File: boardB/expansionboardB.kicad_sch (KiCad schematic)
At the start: 38 parts, among them J1 USB_C_Receptacle, J3 HDMI_A, SW3 ESPRESET, SW4 ESPPROG, U1 ESP32-S3-WROOM-1, U2 GPIO_U2, U4 GPIO_U4, U5 SII1136CTU, U7 MAX20022ATIA+T

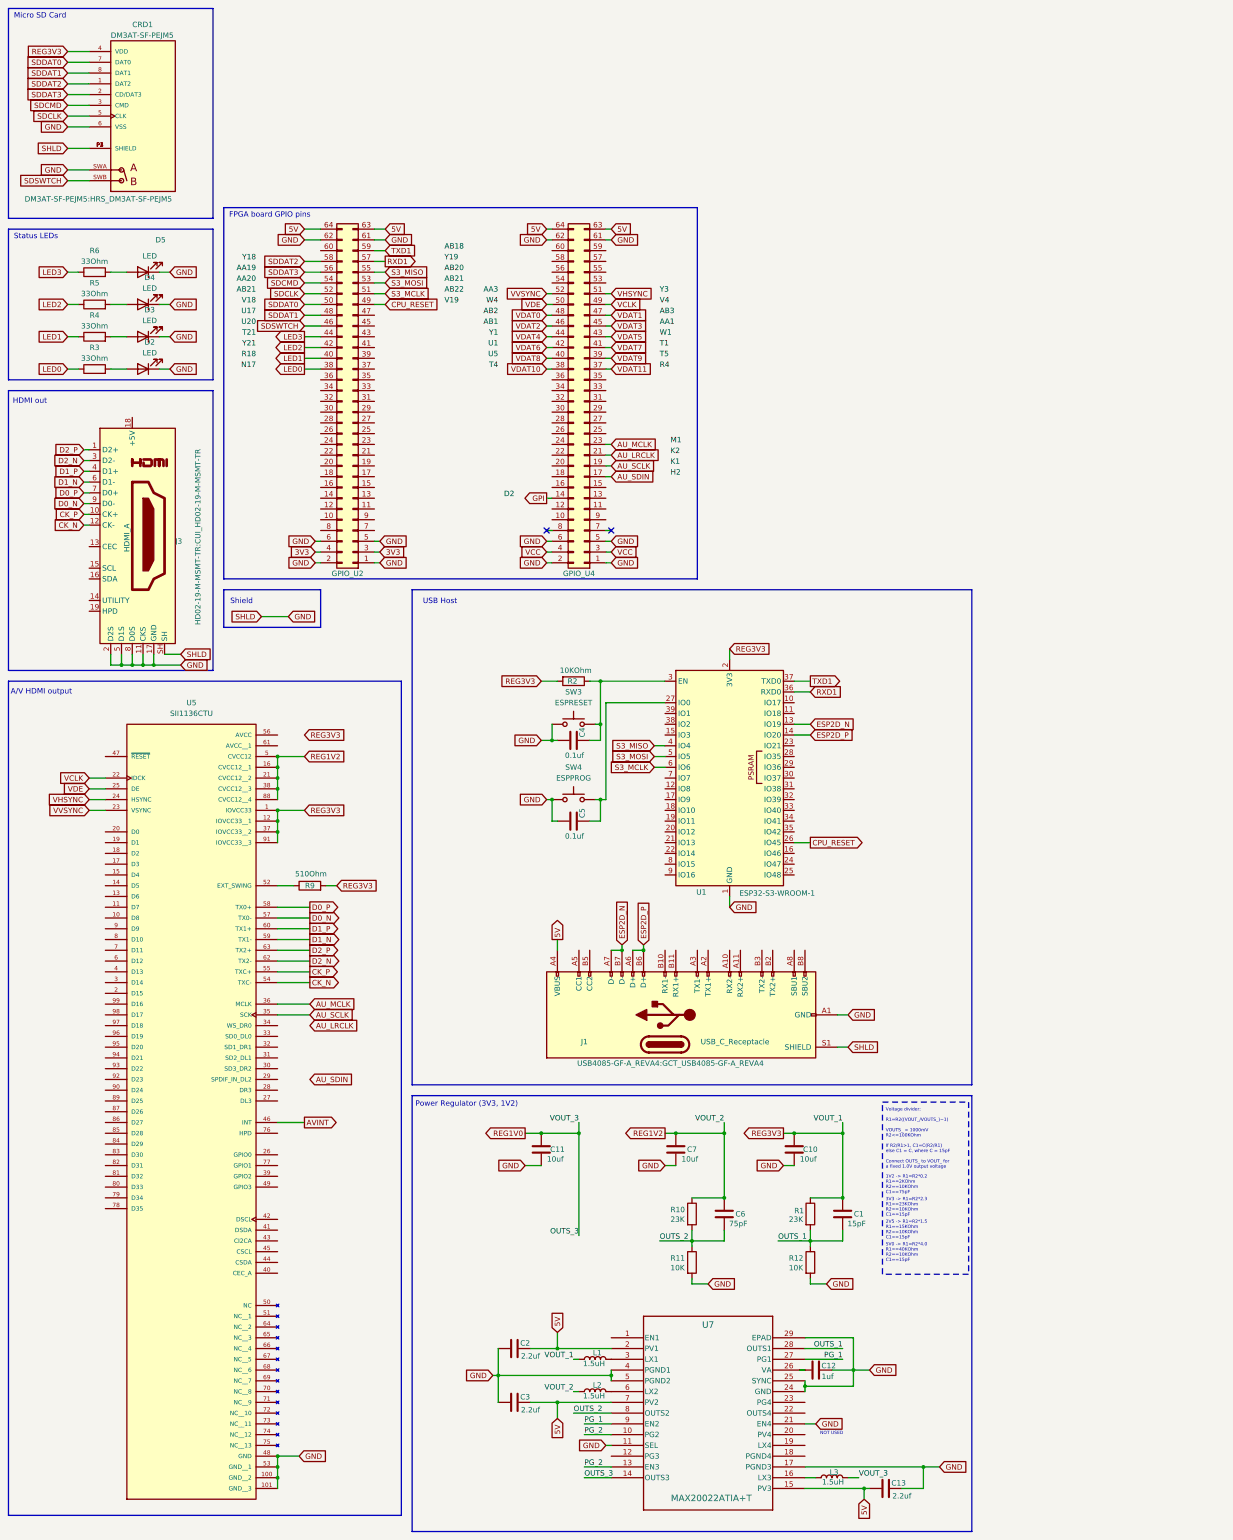
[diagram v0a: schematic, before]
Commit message: Updated new board
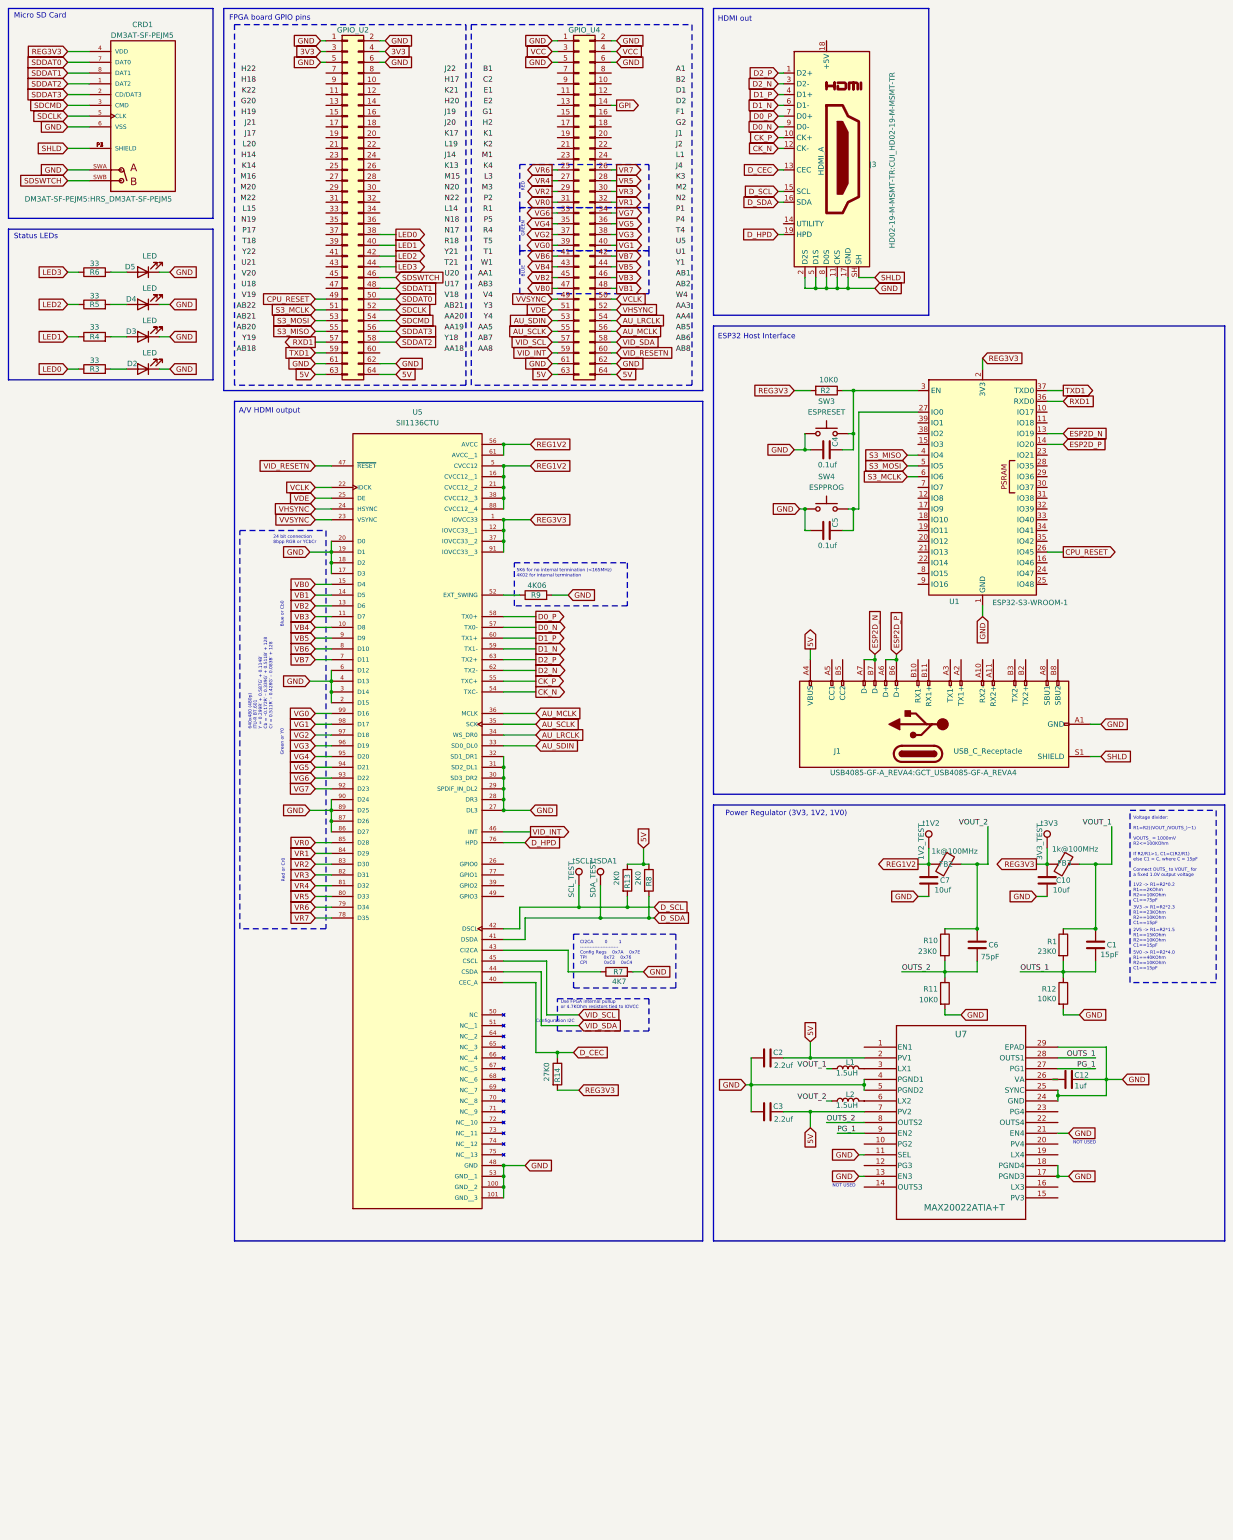
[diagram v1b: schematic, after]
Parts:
- removed C11: 10uf, Capacitor_SMD:C_0603_1608Metric_Pad1.08x0.95mm_HandSolder, symbol Device:C
- removed C13: 2.2uf, Capacitor_SMD:C_0603_1608Metric_Pad1.08x0.95mm_HandSolder, symbol Device:C
- removed L3: 1.5uH, Inductor_SMD:L_0805_2012Metric, symbol Device:L
- added FB2, FB3: 1k@100MHz, Resistor_SMD:R_0805_2012Metric_Pad1.20x1.40mm_HandSolder, symbol graphics-card-rev-2-rescue:Ferrite_Bead-Device
- added R13, R8: 2K0, Resistor_SMD:R_0603_1608Metric_Pad0.98x0.95mm_HandSolder, symbol Device:R
- added R14: 27K0, Resistor_SMD:R_0603_1608Metric_Pad0.98x0.95mm_HandSolder, symbol Device:R
- added R7: 4K7, Resistor_SMD:R_0603_1608Metric_Pad0.98x0.95mm_HandSolder, symbol Device:R
- added t1V2: 1V2_TEST, TestPoint:TestPoint_Pad_D1.5mm, symbol Connector:TestPoint
- added t3V3: 3V3_TEST, TestPoint:TestPoint_Pad_D1.5mm, symbol Connector:TestPoint
- added tSCL1: SCL_TEST, TestPoint:TestPoint_Pad_D1.5mm, symbol Connector:TestPoint
- added tSDA1: SDA_TEST, TestPoint:TestPoint_Pad_D1.5mm, symbol Connector:TestPoint
- R1, R10: value 23K -> 23K0
- R11, R12: value 10K -> 10K0
- R2: value 10KOhm -> 10K0
- R3, R4, R5, R6: value 33Ohm -> 33
- R9: value 510Ohm -> 4K06
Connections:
- net AVINT is gone; now on net VID_INT: U5.46 (INT)
- net VDAT0 is gone; now on net VB1: U4.48 (Pin_48)
- net VDAT1 is gone; now on net VB0: U4.47 (Pin_47)
- net VDAT10 is gone; now on net VG3: U4.38 (Pin_38)
- net VDAT11 is gone; now on net VG2: U4.37 (Pin_37)
- net VDAT2 is gone; now on net VB3: U4.46 (Pin_46)
- net VDAT3 is gone; now on net VB2: U4.45 (Pin_45)
- net VDAT4 is gone; now on net VB5: U4.44 (Pin_44)
- net VDAT5 is gone; now on net VB4: U4.43 (Pin_43)
- net VDAT6 is gone; now on net VB7: U4.42 (Pin_42)
- net VDAT7 is gone; now on net VB6: U4.41 (Pin_41)
- net VDAT8 is gone; now on net VG1: U4.40 (Pin_40)
- net VDAT9 is gone; now on net VG0: U4.39 (Pin_39)
- net 5V: now also R13.1, R8.1; no longer U7.15 (PV3)
- net AU_LRCLK: now also U4.54 (Pin_54), U5.34 (WS_DR0); no longer U4.21 (Pin_21)
- net AU_MCLK: now also U4.56 (Pin_56); no longer U4.23 (Pin_23)
- net AU_SCLK: now also U4.55 (Pin_55); no longer U4.19 (Pin_19)
- net AU_SDIN: now also U4.53 (Pin_53), U5.33 (SD0_DL0); no longer U4.17 (Pin_17)
- net GND: now also R9.2, U5.17 (D3), U5.18 (D2), U5.19 (D1), U5.2 (D15), U5.20 (D0), U5.27 (DL3), U5.28 (DR3), U5.29 (SPDIF_IN_DL2), U5.3 (D14), U5.30 (SD3_DR2), U5.31 (SD2_DL1), U5.32 (SD1_DR1), U5.4 (D13), U5.6 (D12), U5.86 (D27), U5.87 (D26), U5.89 (D25), U5.90 (D24), U7.13 (EN3), U7.18 (PGND4), R7.2; no longer CRD1.P1 (SHIELD), CRD1.P2 (SHIELD), CRD1.P3 (SHIELD), CRD1.P4 (SHIELD), J1.S1 (SHIELD), J3.SH
- net REG1V2: now also U5.56 (AVCC), U5.61 (AVCC__1), FB2.2, t1V2.1; no longer C6.1, L2.1, R10.1
- net REG3V3: now also FB3.2, R14.2, t3V3.1; no longer C1.1, L1.1, R1.1, R9.2
- net VCLK: now also U4.50 (Pin_50); no longer U4.49 (Pin_49)
- net VDE: now also U4.51 (Pin_51); no longer U4.50 (Pin_50)
- net VHSYNC: now also U4.52 (Pin_52); no longer U4.51 (Pin_51)
- net VVSYNC: now also U4.49 (Pin_49); no longer U4.52 (Pin_52)
- net VR6: now reaches U4.25 (Pin_25)
- net VR6: now also U5.79 (D34)
- net VR7: now reaches U4.26 (Pin_26)
- net VR7: now also U5.78 (D35)
- net VR4: now reaches U4.27 (Pin_27)
- net VR4: now also U5.81 (D32)
- net VR5: now reaches U4.28 (Pin_28)
- net VR5: now also U5.80 (D33)
- net VR2: now reaches U4.29 (Pin_29)
- net VR2: now also U5.83 (D30)
- net VR3: now reaches U4.30 (Pin_30)
- net VR3: now also U5.82 (D31)
- net VR0: now reaches U4.31 (Pin_31)
- net VR0: now also U5.85 (D28)
- net VR1: now reaches U4.32 (Pin_32)
- net VR1: now also U5.84 (D29)
- net VG6: now reaches U4.33 (Pin_33)
- net VG6: now also U5.93 (D22)
- net VG7: now reaches U4.34 (Pin_34)
- net VG7: now also U5.92 (D23)
- net VG4: now reaches U4.35 (Pin_35)
- net VG4: now also U5.95 (D20)
- net VG5: now reaches U4.36 (Pin_36)
- net VG5: now also U5.94 (D21)
- net VID_SCL: now reaches U4.57 (Pin_57)
- net VID_SCL: now also U5.45 (CSCL)
- net VID_SDA: now reaches U4.58 (Pin_58)
- net VID_SDA: now also U5.44 (CSDA)
- net VID_INT: now reaches U4.59 (Pin_59)
- net VID_RESETN: now reaches U4.60 (Pin_60)
- net VID_RESETN: now also U5.47 (~{RESET})
- net VB4: now reaches U5.10 (D8)
- net VB3: now reaches U5.11 (D7)
- net VB2: now reaches U5.13 (D6)
- net VB1: now reaches U5.14 (D5)
- net VB0: now reaches U5.15 (D4)
- net D_CEC: now reaches U5.40 (CEC_A)
- net D_CEC: now also J3.13 (CEC), R14.1
- net D_SDA: now reaches U5.41 (DSDA)
- net D_SDA: now also J3.16 (SDA), R8.2, tSDA1.1
- net D_SCL: now reaches U5.42 (DSCL)
- net D_SCL: now also J3.15 (SCL), R13.2, tSCL1.1
- net at U5.43 (CI2CA): now also R7.1
- net VB7: now reaches U5.7 (D11)
- net D_HPD: now reaches U5.76 (HPD)
- net D_HPD: now also J3.19 (HPD)
- net VB6: now reaches U5.8 (D10)
- net VB5: now reaches U5.9 (D9)
- net VG3: now reaches U5.96 (D19)
- net VG2: now reaches U5.97 (D18)
- net VG1: now reaches U5.98 (D17)
- net VG0: now reaches U5.99 (D16)
- net PG_2: no longer names the net of U7.10 (PG2)
- net PG_2: no longer U7.13 (EN3)
- net REG1V0: no longer names the net of U7.14 (OUTS3)
- new net SHLD: CRD1.P1 (SHIELD), CRD1.P2 (SHIELD), CRD1.P3 (SHIELD), CRD1.P4 (SHIELD), J1.S1 (SHIELD), J3.SH
- new net VOUT_1: C1.1, FB3.1, L1.1, R1.1
- new net VOUT_2: C6.1, FB2.1, L2.1, R10.1
- no-connect marks 2 -> 0
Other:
- note added: "24 bit connection 8bpp RGB or YCbCr"
- note added: "5K6 for no internal termination (<165MHz) 4K02 for internal termination"
- note added: "640x480 (480p) ITU-R BT.601 Y = 0.299R′ + 0.587G′ + 0.114B′ Cb = –0.172R′ – 0.339G′ + 0.511B′ + 128 Cr = 0.511R′ – 0.428G′ – 0.083B′ + 128"
- note added: "BLUE"
- note added: "Blue or Cb0"
- note added: "CI2CA 0 1 ------------------------ Config Regs 0x7A 0x7E TPI 0x72 0x76 CPI 0xC0 0xC4"
- note added: "Configuration I2C"
- note added: "ESP32 Host Interface"
- note added: "GREEN"
- note added: "Green or Y0"
- note added: "Power Regulator (3V3, 1V2, 1V0)"
- note added: "RED"
- note added: "Red or Cr0"
- note added: "Use FPGA internal pullup or 4.7KOhm resistors tied to IOVCC"
- note removed: "Power Regulator (3V3, 1V2)"
- note removed: "Shield"
- note removed: "USB Host"
- moved on the sheet: C1, C10, C12, C2, C3, C4, C5, C6, C7, J1, J3, L1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
